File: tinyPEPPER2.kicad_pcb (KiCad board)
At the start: 4 copper layers, 20 x 20 mm, 163 parts, among them T201 BC847, T202 BC847, T203 BC847, T301 BC847, T302 BC847, T303 BC847, T401 BC847, T402 BC847, T403 BC847, T501 BC847, T502 BC847, T503 BC847, U1 AP131-30, U201 EFM8BB10, U301 EFM8BB10, U401 EFM8BB10, U501 EFM8BB10

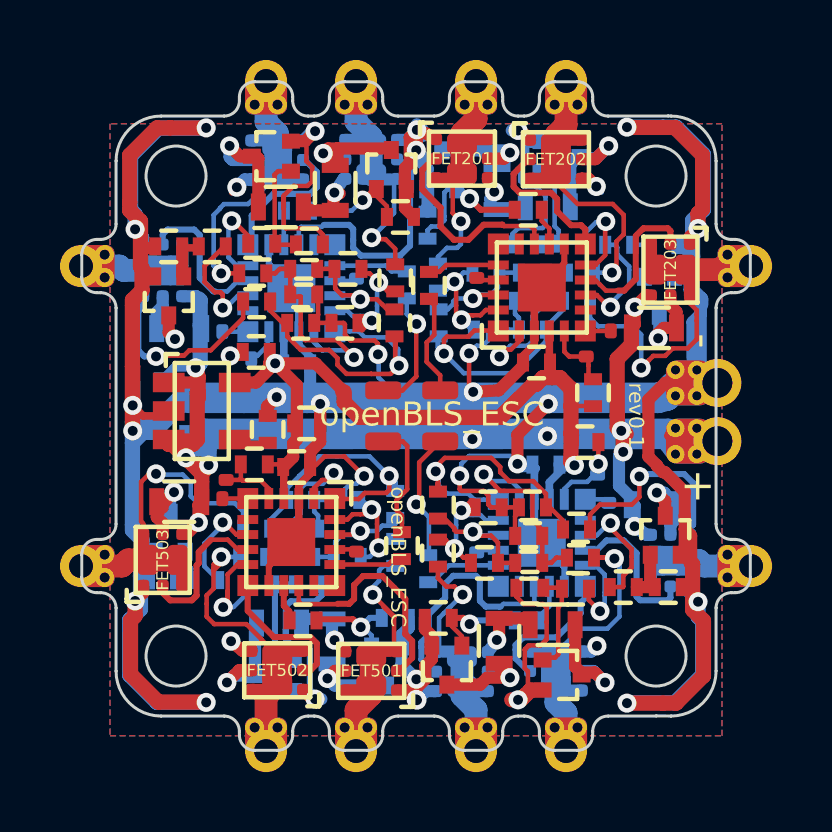
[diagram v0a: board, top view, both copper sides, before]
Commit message: fix symbols table
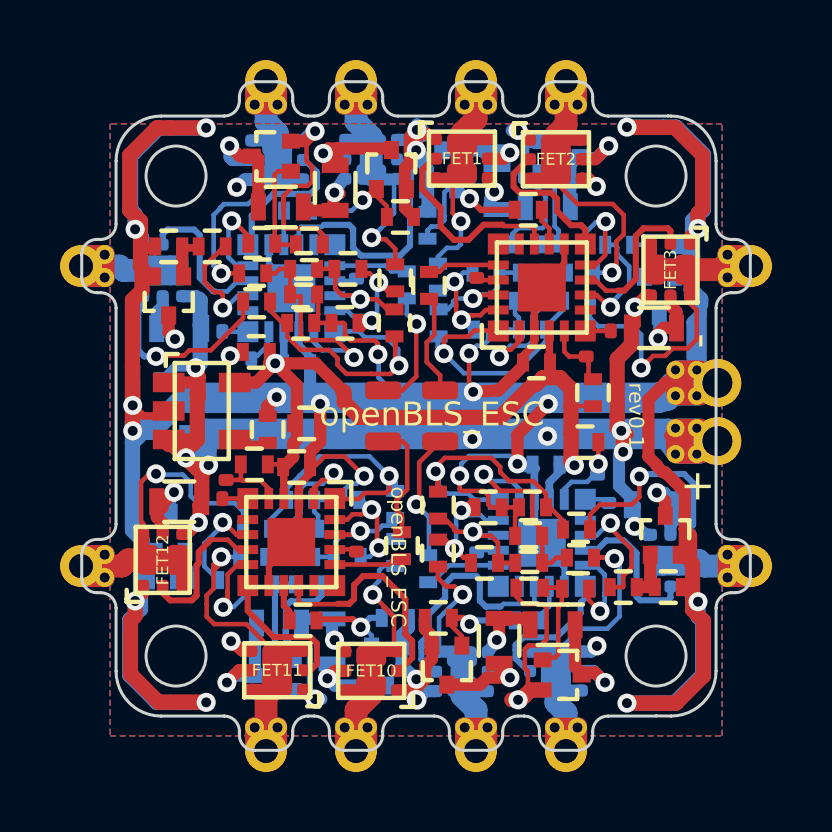
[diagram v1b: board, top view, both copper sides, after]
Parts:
- renumbered BL_TX201 to BL_TX1, BL_TX301 to BL_TX2, BL_TX401 to BL_TX3, BL_TX501 to BL_TX4, C1002 to C1, C302 to C10, C303 to C11, C304 to C12, C401 to C13, C402 to C14, C403 to C15, C404 to C16, C501 to C17, C502 to C18, C503 to C19, C1000 to C2, C504 to C20, C1003 to C3, C1001 to C4, C201 to C5, C202 to C6, C203 to C7, C204 to C8, C301 to C9, FET201 to FET1, FET501 to FET10, FET502 to FET11, FET503 to FET12, FET202 to FET2, FET203 to FET3, FET301 to FET4, FET302 to FET5, FET303 to FET6, FET401 to FET7, FET402 to FET8, FET403 to FET9, OUT_A201 to OUT_A1, OUT_A301 to OUT_A2, OUT_A401 to OUT_A3, OUT_A501 to OUT_A4, OUT_B201 to OUT_B1, OUT_B301 to OUT_B2, OUT_B401 to OUT_B3, OUT_B501 to OUT_B4, OUT_C201 to OUT_C1, OUT_C301 to OUT_C2, OUT_C401 to OUT_C3, OUT_C501 to OUT_C4, R201 to R1, R219 to R10, R214 to R11, R202 to R12, R203 to R13, R204 to R14, R205 to R15, R206 to R16, R207 to R17, R208 to R18, R209 to R19, R220 to R2, R210 to R20, R301 to R21, R320 to R22, R311 to R23, R312 to R24, R313 to R25, R315 to R26, R316 to R27, R317 to R28, R318 to R29, R211 to R3, R319 to R30, R314 to R31, R302 to R32, R303 to R33, R304 to R34, R305 to R35, R306 to R36, R307 to R37, R308 to R38, R309 to R39, R212 to R4, R310 to R40, R401 to R41, R420 to R42, R411 to R43, R412 to R44, R413 to R45, R415 to R46, R416 to R47, R417 to R48, R418 to R49, R213 to R5, R419 to R50, R414 to R51, R402 to R52, R403 to R53, R404 to R54, R405 to R55, R406 to R56, R407 to R57, R408 to R58, R409 to R59, R215 to R6, R410 to R60, R501 to R61, R520 to R62, R511 to R63, R512 to R64, R513 to R65, R515 to R66, R516 to R67, R517 to R68, R518 to R69, R216 to R7, R519 to R70, R514 to R71, R502 to R72, R503 to R73, R504 to R74, R505 to R75, R506 to R76, R507 to R77, R508 to R78, R509 to R79, R217 to R8, R510 to R80, R218 to R9, T201 to T1, T501 to T10, T502 to T11, T503 to T12, T202 to T2, T203 to T3, T301 to T4, T302 to T5, T303 to T6, T401 to T7, T402 to T8, T403 to T9, TP10 to TP1, TP302 to TP10, TP403 to TP11, TP402 to TP12, TP503 to TP13, TP502 to TP14, TP12 to TP2, TP103 to TP3, TP104 to TP4, TP105 to TP5, TP106 to TP6, TP203 to TP7, TP202 to TP8, TP303 to TP9, U201 to U2, U301 to U3, U401 to U4, U501 to U5
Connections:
- net /single esc 3/RC_IN renamed /single esc 3/RC_IN_0
- net /single esc 4/RC_IN renamed /single esc 4/RC_IN_0
- R12 pad 1: Net-(R202-Pad1) -> Net-(R12-~-Pad1)
- R12 pad 2: Net-(R202-Pad2) -> Net-(R12-~-Pad2)
- R13 pad 1: Net-(R202-Pad2) -> Net-(R12-~-Pad2)
- R14 pad 1: Net-(R202-Pad1) -> Net-(U2-P0.3)
- R14 pad 2: Net-(R204-Pad2) -> Net-(R14-~-Pad2)
- R15 pad 1: Net-(R204-Pad2) -> Net-(R14-~-Pad2)
- R16 pad 1: Net-(R202-Pad1) -> Net-(R12-~-Pad1)
- R16 pad 2: Net-(R206-Pad2) -> Net-(R16-~-Pad2)
- R17 pad 1: Net-(R206-Pad2) -> Net-(R16-~-Pad2)
- R18 pad 2: Net-(R202-Pad2) -> Net-(U2-P0.2)
- R19 pad 2: Net-(R204-Pad2) -> Net-(U2-P0.0)
- R20 pad 2: Net-(R206-Pad2) -> Net-(U2-P0.1)
- R32 pad 1: Net-(R302-Pad1) -> Net-(R32-~-Pad1)
- R32 pad 2: Net-(R302-Pad2) -> Net-(R32-~-Pad2)
- R33 pad 1: Net-(R302-Pad2) -> Net-(R32-~-Pad2)
- R34 pad 1: Net-(R302-Pad1) -> Net-(U3-P0.3)
- R34 pad 2: Net-(R304-Pad2) -> Net-(R34-~-Pad2)
- R35 pad 1: Net-(R304-Pad2) -> Net-(R34-~-Pad2)
- R36 pad 1: Net-(R302-Pad1) -> Net-(R32-~-Pad1)
- R36 pad 2: Net-(R306-Pad2) -> Net-(R36-~-Pad2)
- R37 pad 1: Net-(R306-Pad2) -> Net-(R36-~-Pad2)
- R38 pad 2: Net-(R302-Pad2) -> Net-(U3-P0.2)
- R39 pad 2: Net-(R304-Pad2) -> Net-(U3-P0.0)
- R40 pad 2: Net-(R306-Pad2) -> Net-(U3-P0.1)
- R52 pad 1: Net-(R402-Pad1) -> Net-(R52-~-Pad1)
- R52 pad 2: Net-(R402-Pad2) -> Net-(R52-~-Pad2)
- R53 pad 1: Net-(R402-Pad2) -> Net-(R52-~-Pad2)
- R54 pad 1: Net-(R402-Pad1) -> Net-(U4-P0.3)
- R54 pad 2: Net-(R404-Pad2) -> Net-(R54-~-Pad2)
- R55 pad 1: Net-(R404-Pad2) -> Net-(R54-~-Pad2)
- R56 pad 1: Net-(R402-Pad1) -> Net-(R52-~-Pad1)
- R56 pad 2: Net-(R406-Pad2) -> Net-(R56-~-Pad2)
- R57 pad 1: Net-(R406-Pad2) -> Net-(R56-~-Pad2)
- R58 pad 2: Net-(R402-Pad2) -> Net-(U4-P0.2)
- R59 pad 2: Net-(R404-Pad2) -> Net-(U4-P0.0)
- R60 pad 2: Net-(R406-Pad2) -> Net-(U4-P0.1)
- R72 pad 1: Net-(R502-Pad1) -> Net-(R72-~-Pad1)
- R72 pad 2: Net-(R502-Pad2) -> Net-(R72-~-Pad2)
- R73 pad 1: Net-(R502-Pad2) -> Net-(R72-~-Pad2)
- R74 pad 1: Net-(R502-Pad1) -> Net-(U5-P0.3)
- R74 pad 2: Net-(R504-Pad2) -> Net-(R74-~-Pad2)
- R75 pad 1: Net-(R504-Pad2) -> Net-(R74-~-Pad2)
- R76 pad 1: Net-(R502-Pad1) -> Net-(R72-~-Pad1)
- R76 pad 2: Net-(R506-Pad2) -> Net-(R76-~-Pad2)
- R77 pad 1: Net-(R506-Pad2) -> Net-(R76-~-Pad2)
- R78 pad 2: Net-(R502-Pad2) -> Net-(U5-P0.2)
- R79 pad 2: Net-(R504-Pad2) -> Net-(U5-P0.0)
- R80 pad 2: Net-(R506-Pad2) -> Net-(U5-P0.1)
- U2 pad 1: Net-(R206-Pad2) -> Net-(U2-P0.1)
- U2 pad 15: (no net) -> unconnected-(U2-P0.7-Pad15)
- U2 pad 16: (no net) -> unconnected-(U2-P0.6-Pad16)
- U2 pad 19: Net-(R202-Pad1) -> Net-(U2-P0.3)
- U2 pad 2: Net-(R204-Pad2) -> Net-(U2-P0.0)
- U2 pad 20: Net-(R202-Pad2) -> Net-(U2-P0.2)
- U2 pad 7: (no net) -> unconnected-(U2-P1.6-Pad7)
- U3 pad 1: Net-(R306-Pad2) -> Net-(U3-P0.1)
- U3 pad 15: (no net) -> unconnected-(U3-P0.7-Pad15)
- U3 pad 16: (no net) -> unconnected-(U3-P0.6-Pad16)
- U3 pad 19: Net-(R302-Pad1) -> Net-(U3-P0.3)
- U3 pad 2: Net-(R304-Pad2) -> Net-(U3-P0.0)
- U3 pad 20: Net-(R302-Pad2) -> Net-(U3-P0.2)
- U3 pad 7: (no net) -> unconnected-(U3-P1.6-Pad7)
- U4 pad 1: Net-(R406-Pad2) -> Net-(U4-P0.1)
- U4 pad 15: (no net) -> unconnected-(U4-P0.7-Pad15)
- U4 pad 16: (no net) -> unconnected-(U4-P0.6-Pad16)
- U4 pad 19: Net-(R402-Pad1) -> Net-(U4-P0.3)
- U4 pad 2: Net-(R404-Pad2) -> Net-(U4-P0.0)
- U4 pad 20: Net-(R402-Pad2) -> Net-(U4-P0.2)
- U4 pad 7: (no net) -> unconnected-(U4-P1.6-Pad7)
- U5 pad 1: Net-(R506-Pad2) -> Net-(U5-P0.1)
- U5 pad 15: (no net) -> unconnected-(U5-P0.7-Pad15)
- U5 pad 16: (no net) -> unconnected-(U5-P0.6-Pad16)
- U5 pad 19: Net-(R502-Pad1) -> Net-(U5-P0.3)
- U5 pad 2: Net-(R504-Pad2) -> Net-(U5-P0.0)
- U5 pad 20: Net-(R502-Pad2) -> Net-(U5-P0.2)
- U5 pad 7: (no net) -> unconnected-(U5-P1.6-Pad7)
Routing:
- net (no net): track 0.00 -> 104.2 mm, vias 0 -> 20
- net Net-(R306-Pad2): track 11.1 -> 0.00 mm, vias 1 -> 0
- net Net-(R406-Pad2): track 10.6 -> 0.00 mm, vias 1 -> 0
- net Net-(R506-Pad2): track 9.35 -> 0.00 mm, vias 1 -> 0
- net Net-(R206-Pad2): track 9.34 -> 0.00 mm, vias 1 -> 0
- net Net-(R304-Pad2): track 8.10 -> 0.00 mm, vias 1 -> 0
- net Net-(R404-Pad2): track 7.08 -> 0.00 mm, vias 1 -> 0
- net Net-(R204-Pad2): track 5.74 -> 0.00 mm, vias 1 -> 0
- net Net-(R504-Pad2): track 5.70 -> 0.00 mm, vias 1 -> 0
- net Net-(R202-Pad1): track 4.80 -> 0.00 mm, vias 1 -> 0
- net Net-(R502-Pad1): track 4.72 -> 0.00 mm, vias 1 -> 0
- net Net-(R502-Pad2): track 4.69 -> 0.00 mm, vias 2 -> 0
- net Net-(R202-Pad2): track 4.69 -> 0.00 mm, vias 2 -> 0
- net Net-(R402-Pad2): track 4.69 -> 0.00 mm, vias 2 -> 0
- net Net-(R302-Pad1): track 4.64 -> 0.00 mm, vias 1 -> 0
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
